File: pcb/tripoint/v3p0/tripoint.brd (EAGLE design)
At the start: 30.5 x 16.4 mm, 72 parts, among them J2 TC2030-JLINK-NL, T1 HHM1595A1, U1 STM32F091CC, U2 DW1000, U3 SKY13317, U4 LXDC2HN18A, X1 38.4M, X2 16M

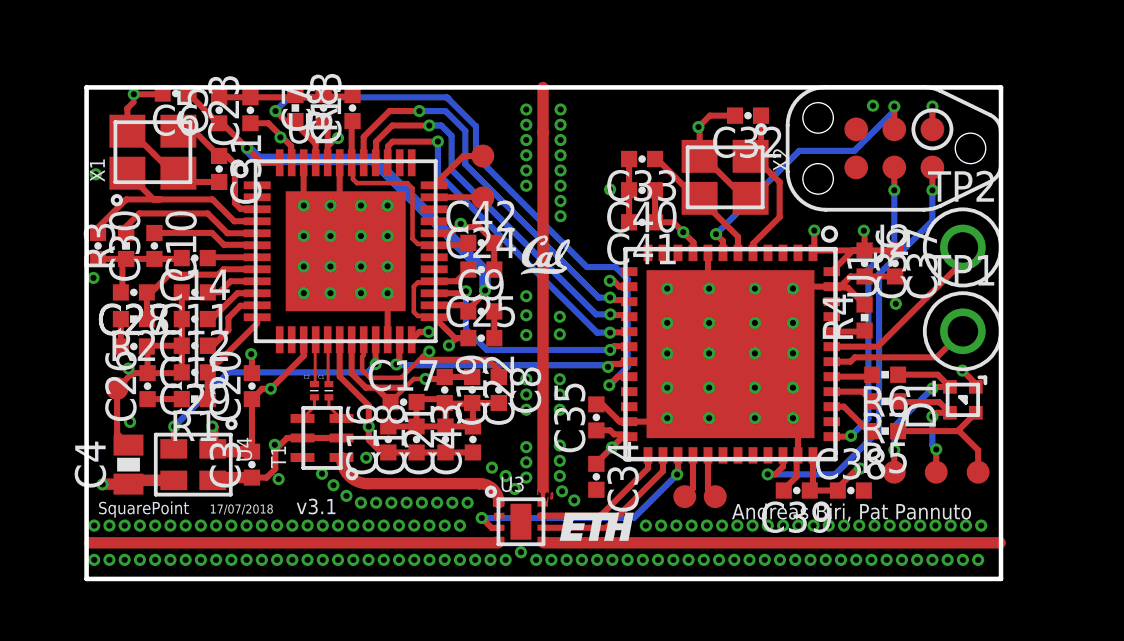
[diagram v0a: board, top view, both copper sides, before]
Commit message: finished silk for SquarePoint
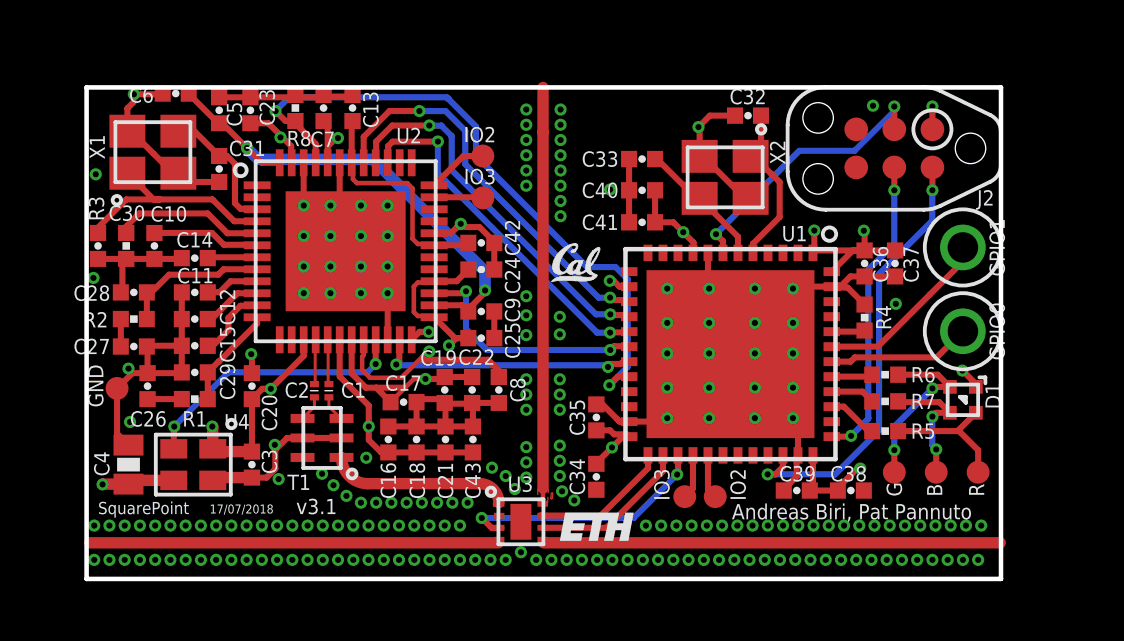
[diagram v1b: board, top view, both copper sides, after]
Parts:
- moved U$2 1.05 mm to (0.25, 4.06)
- renumbered TP1 to GPIO0, TP2 to GPIO1
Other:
- board text added: "B"
- board text added: "G"
- board text added: "GND"
- board text added: "IO2"
- board text added: "IO3"
- board text added: "R"
